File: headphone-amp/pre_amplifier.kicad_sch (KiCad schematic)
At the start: 4 parts, among them U701 NE5532

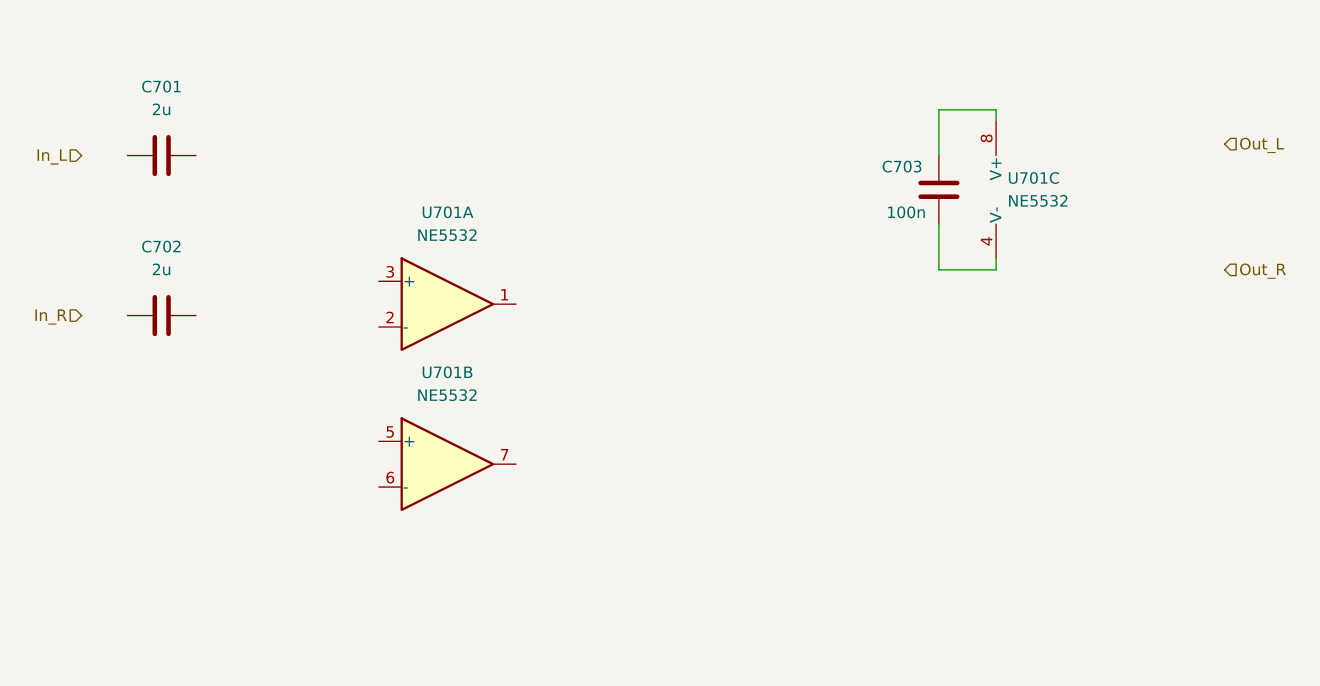
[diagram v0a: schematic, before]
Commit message: Updated headphone-amp kicad project
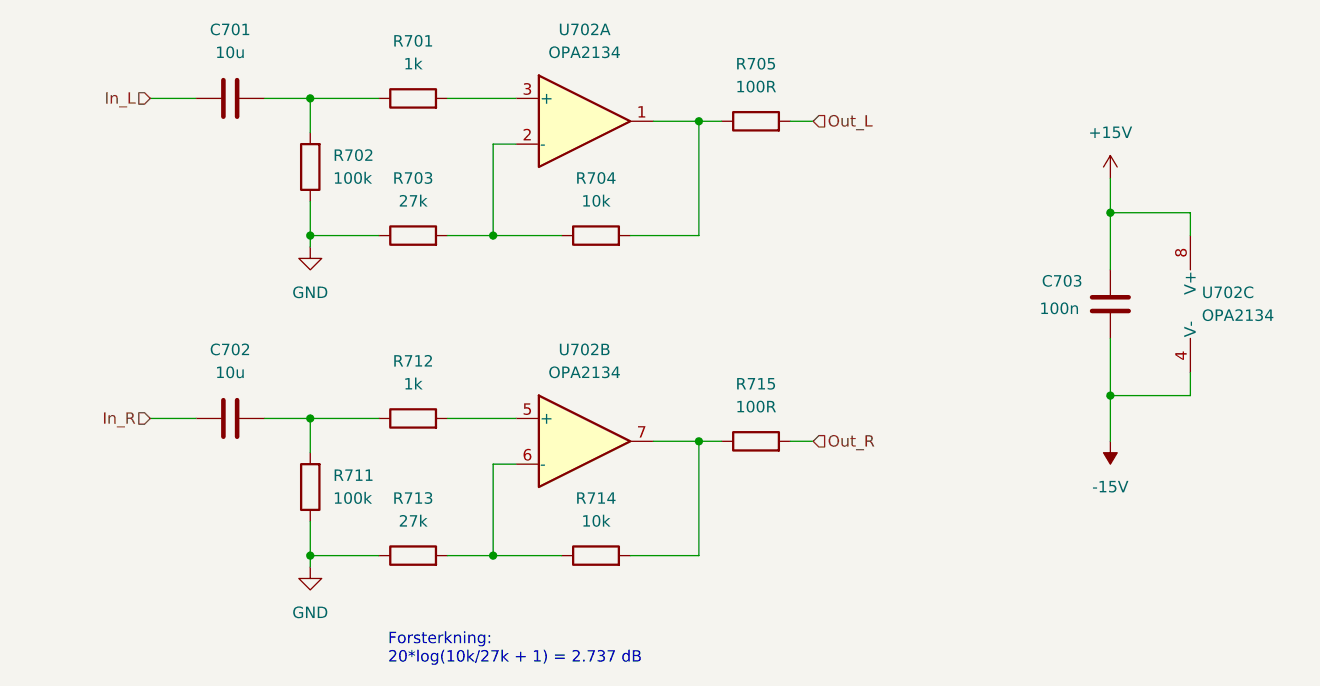
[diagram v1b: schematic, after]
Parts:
- removed U701: NE5532, Package_DIP:DIP-8_W7.62mm_LongPads, symbol Amplifier_Operational:NE5532
- added R701, R712: 1k, Resistor_THT:R_Axial_DIN0207_L6.3mm_D2.5mm_P10.16mm_Horizontal, symbol Device:R
- added R702, R711: 100k, Resistor_THT:R_Axial_DIN0207_L6.3mm_D2.5mm_P10.16mm_Horizontal, symbol Device:R
- added R703, R713: 27k, Resistor_THT:R_Axial_DIN0207_L6.3mm_D2.5mm_P10.16mm_Horizontal, symbol Device:R
- added R704, R714: 10k, Resistor_THT:R_Axial_DIN0207_L6.3mm_D2.5mm_P10.16mm_Horizontal, symbol Device:R
- added R705, R715: 100R, Resistor_THT:R_Axial_DIN0207_L6.3mm_D2.5mm_P10.16mm_Horizontal, symbol Device:R
- added U702: OPA2134, Package_DIP:DIP-8_W7.62mm_LongPads, symbol Amplifier_Operational:OPA2134
- C701, C702: value 2u -> 10u
- C703: footprint Capacitor_THT:C_Axial_L12.0mm_D7.5mm_P15.00mm_Horizontal -> Capacitor_THT:C_Disc_D6.0mm_W2.5mm_P5.00mm
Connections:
- net In_L: now also C701.1
- net In_R: now also C702.1
- net Out_L: now also R705.2
- net Out_R: now also R715.2
- net +15V: now reaches C703.1
- net +15V: now also U702.8 (V+)
- net -15V: now reaches C703.2
- net -15V: now also U702.4 (V-)
- net at C702.2: now also R711.2, R712.1
- net at C701.2: now also R701.1, R702.2
- new net: R712.2, U702.5 (+)
- new net: R704.2, R705.1, U702.1
- new net: R703.2, R704.1, U702.2 (-)
- new net: R701.2, U702.3 (+)
- new net: R713.2, R714.1, U702.6 (-)
- new net: R714.2, R715.1, U702.7
- new net GND: R702.1, R703.1, R711.1, R713.1
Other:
- note added: "Forsterkning: 20*log(10k/27k + 1) = 2.737 dB"
- moved on the sheet: C701
